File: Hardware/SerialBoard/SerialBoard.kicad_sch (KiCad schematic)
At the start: 10 parts, among them J1 PORT1, J2 DATA, J3 CTRL, J4 CTRL, J5 DATA, U1 W65C51N, Y1 1.8432MHz

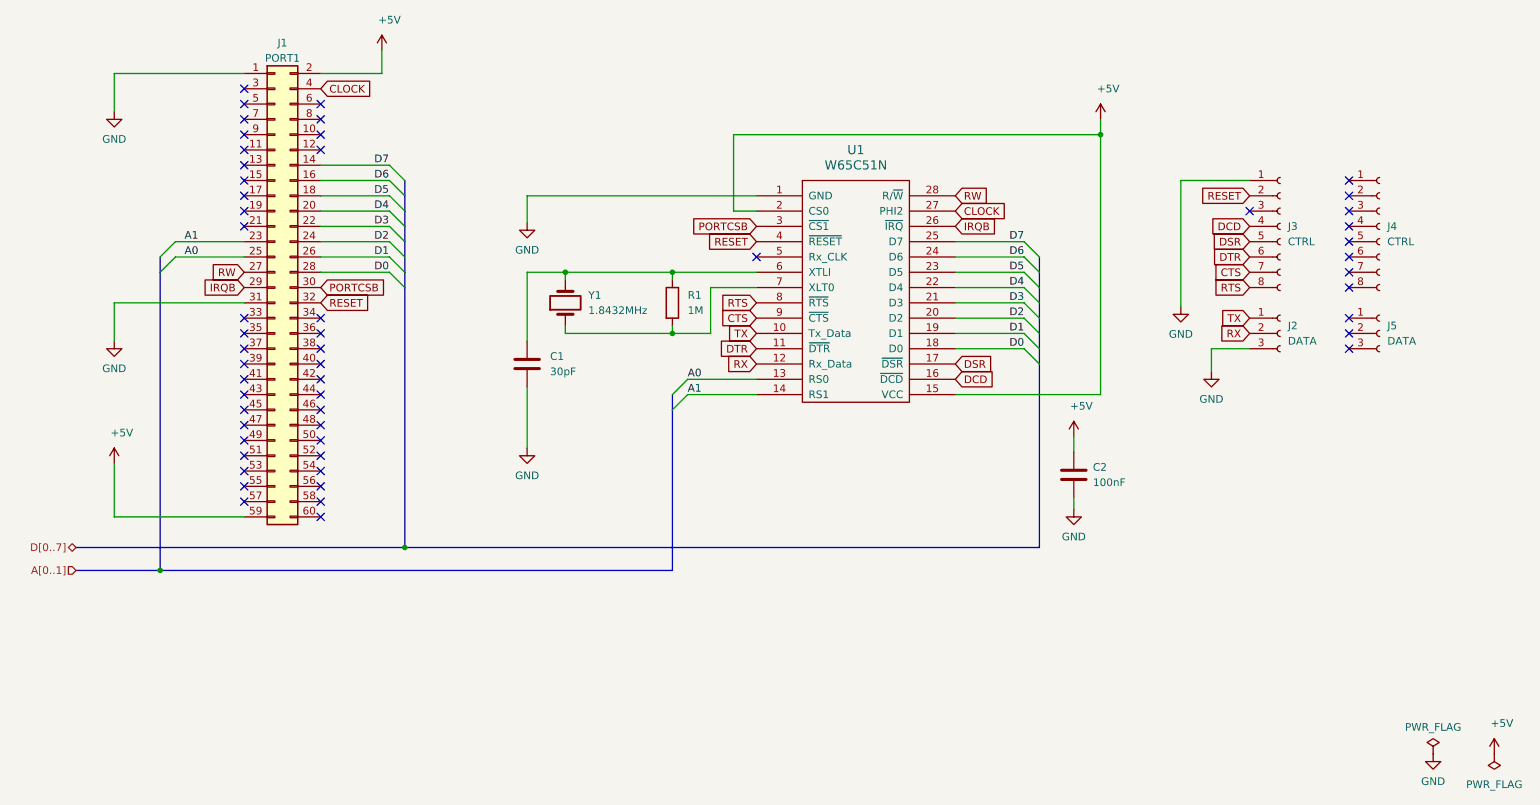
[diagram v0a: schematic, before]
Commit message: Fix
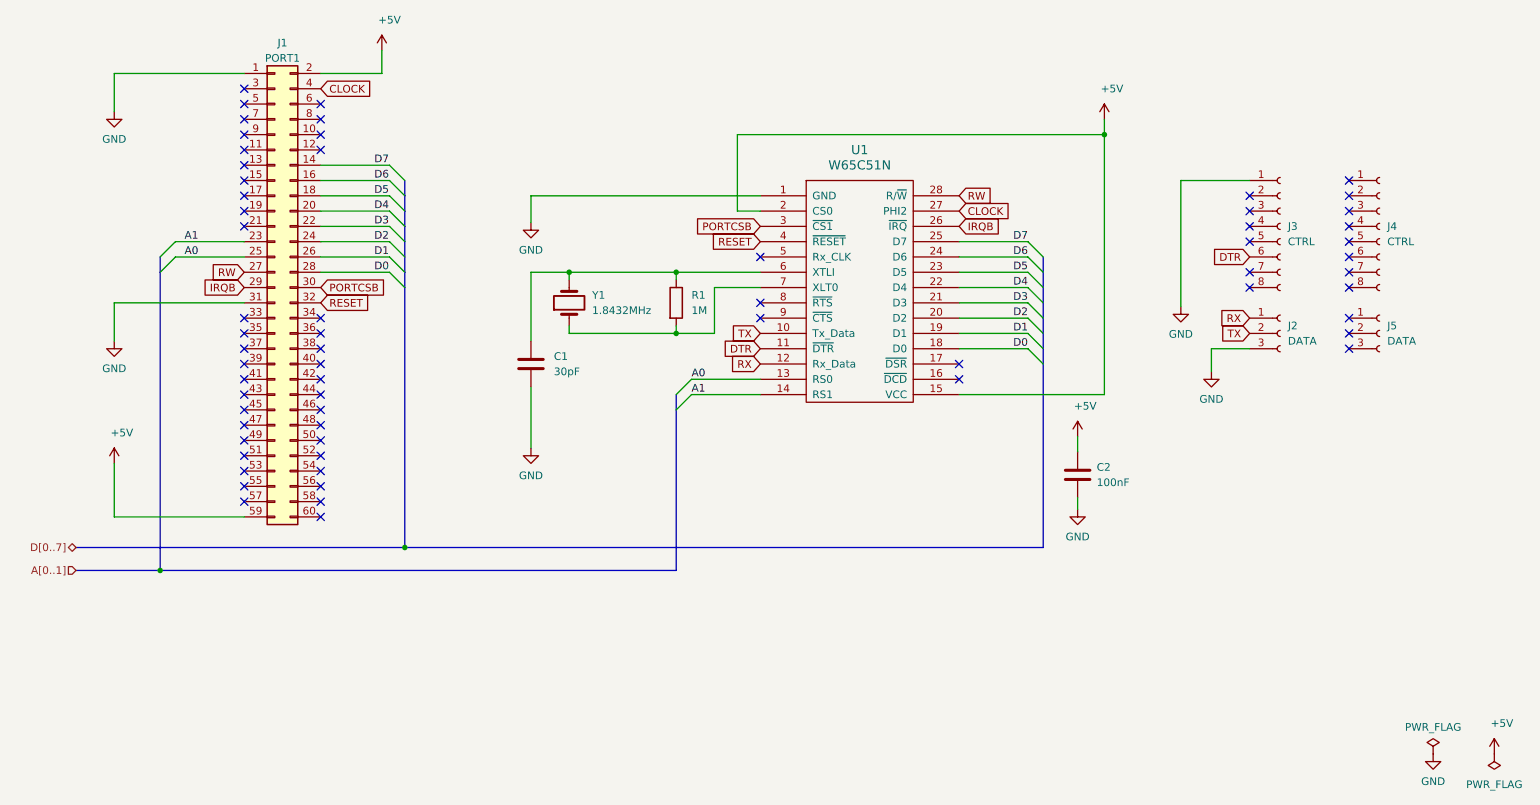
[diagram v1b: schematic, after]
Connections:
- net RESET: no longer J3.2 (Pin_2)
- net RX: now also J2.1 (Pin_1); no longer J2.2 (Pin_2)
- net TX: now also J2.2 (Pin_2); no longer J2.1 (Pin_1)
- net CTS: no longer names the net of U1.9 (~{CTS})
- net CTS: no longer J3.7 (Pin_7)
- net DCD: no longer names the net of U1.16 (~{DCD})
- net DCD: no longer J3.4 (Pin_4)
- net DSR: no longer names the net of U1.17 (~{DSR})
- net DSR: no longer J3.5 (Pin_5)
- net RTS: no longer names the net of U1.8 (~{RTS})
- net RTS: no longer J3.8 (Pin_8)
- no-connect marks 54 -> 63
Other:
- moved on the sheet: C1, C2, R1, U1, Y1
